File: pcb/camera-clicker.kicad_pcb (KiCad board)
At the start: 2 copper layers, 28 x 106.3 mm, 32 parts, among them J1 USB_C_Receptacle_USB2.0, J2 Conn_01x06, SW1 SW_SPST, SW2 BOOT, SW3 RST, SW4 SW_DPST_x2, U2 ESP32-MINI-1, U3 MCP2221AxST, U4 AZ1117-3.3

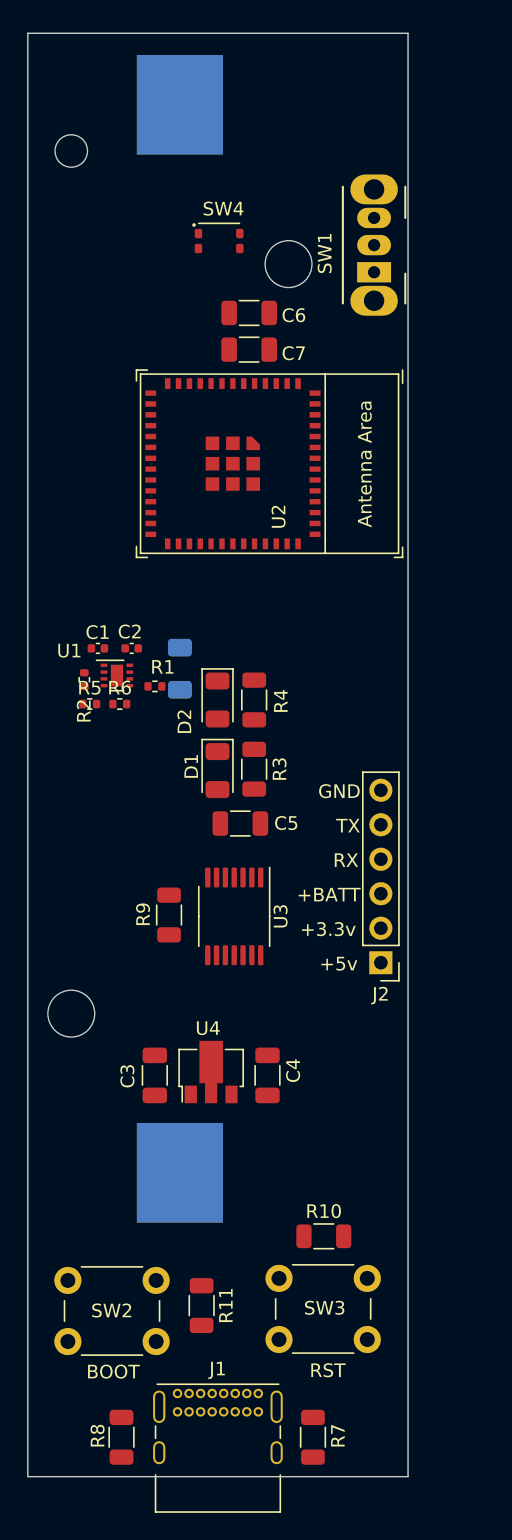
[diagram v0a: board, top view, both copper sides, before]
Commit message: fixing position
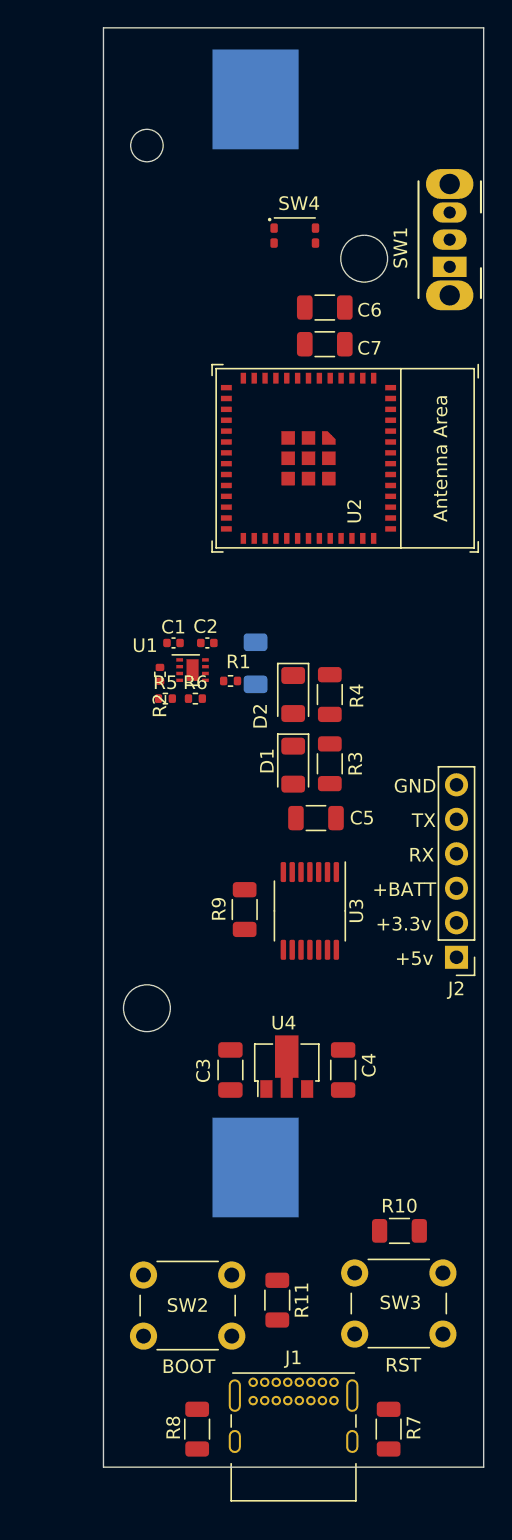
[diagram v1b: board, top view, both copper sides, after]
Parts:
- moved J1 5.63 mm to (141.0, 141.8)
- moved R7 5.60 mm to (151.0, 145.2)
- moved R8 5.60 mm to (136.9, 145.2)
- moved C7 5.58 mm to (146.3, 65.3)
- moved R1 5.58 mm to (139.4, 90.1)
- moved R10 5.58 mm to (151.8, 130.6)
- moved R11 5.58 mm to (142.8, 135.7)
- moved C6 5.58 mm to (146.3, 62.6)
- moved R6 5.58 mm to (136.8, 91.4)
- moved BT1 5.58 mm to (141.2, 86.6)
- moved C1 5.58 mm to (135.2, 87.3)
- moved C2 5.58 mm to (137.7, 87.3)
- moved C3 5.58 mm to (139.3, 118.8)
- moved C4 5.58 mm to (147.7, 118.8)
- moved D1 5.58 mm to (144.0, 96.3)
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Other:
- board size 28 x 106.3 mm -> 28 x 106 mm
